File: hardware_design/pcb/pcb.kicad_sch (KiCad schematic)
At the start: 15 parts, among them J1 Eurorack Power, Q1 DMG2305UX, U1 Pico, U2 PCM1808, U5 GY_PCM5102A, U6 APS6404L, U7 LM1117MP-5.0

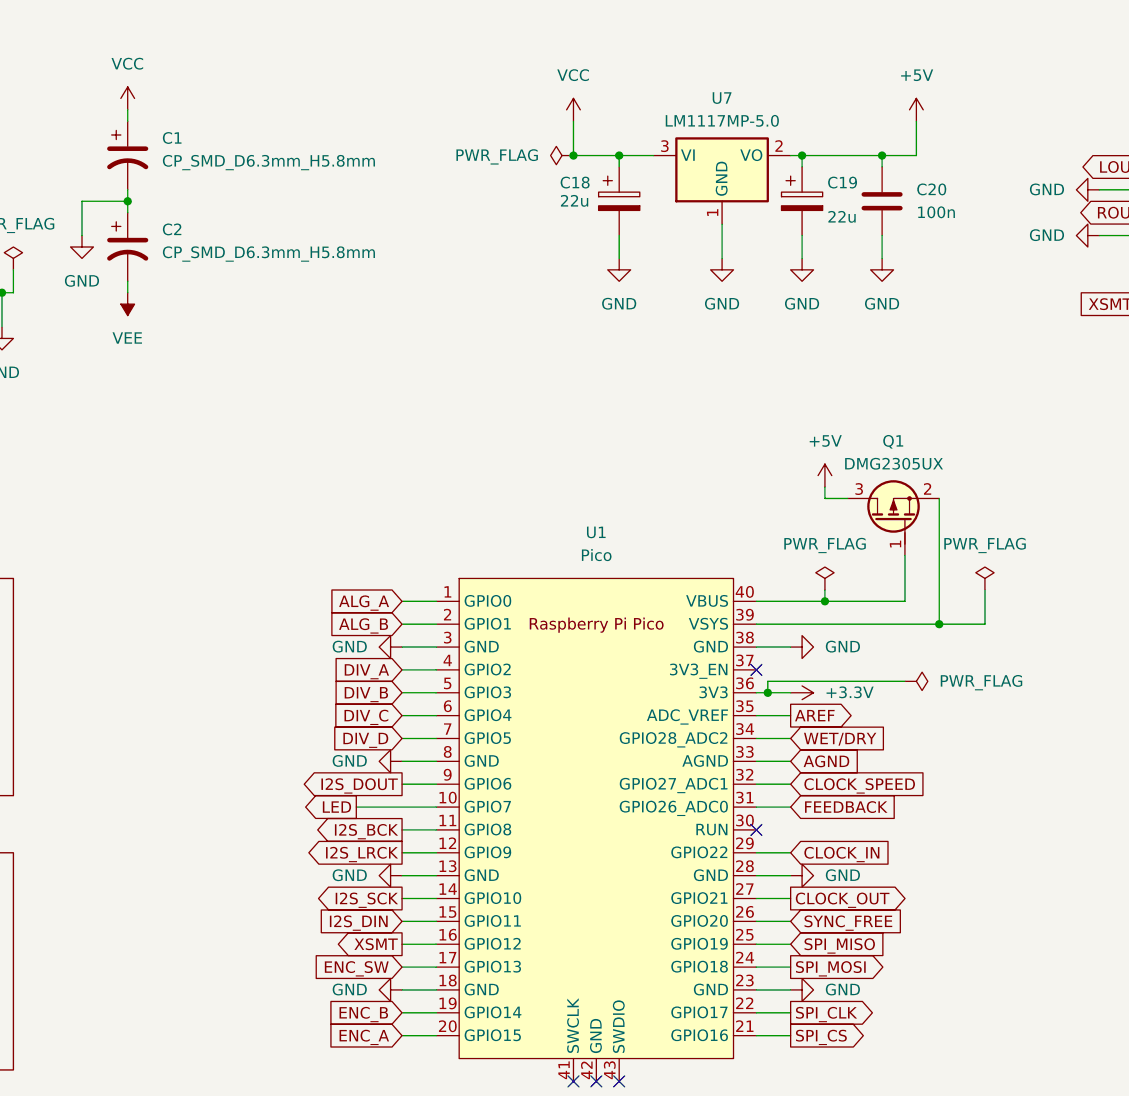
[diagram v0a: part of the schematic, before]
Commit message: Rev 2 schematic & circuit board
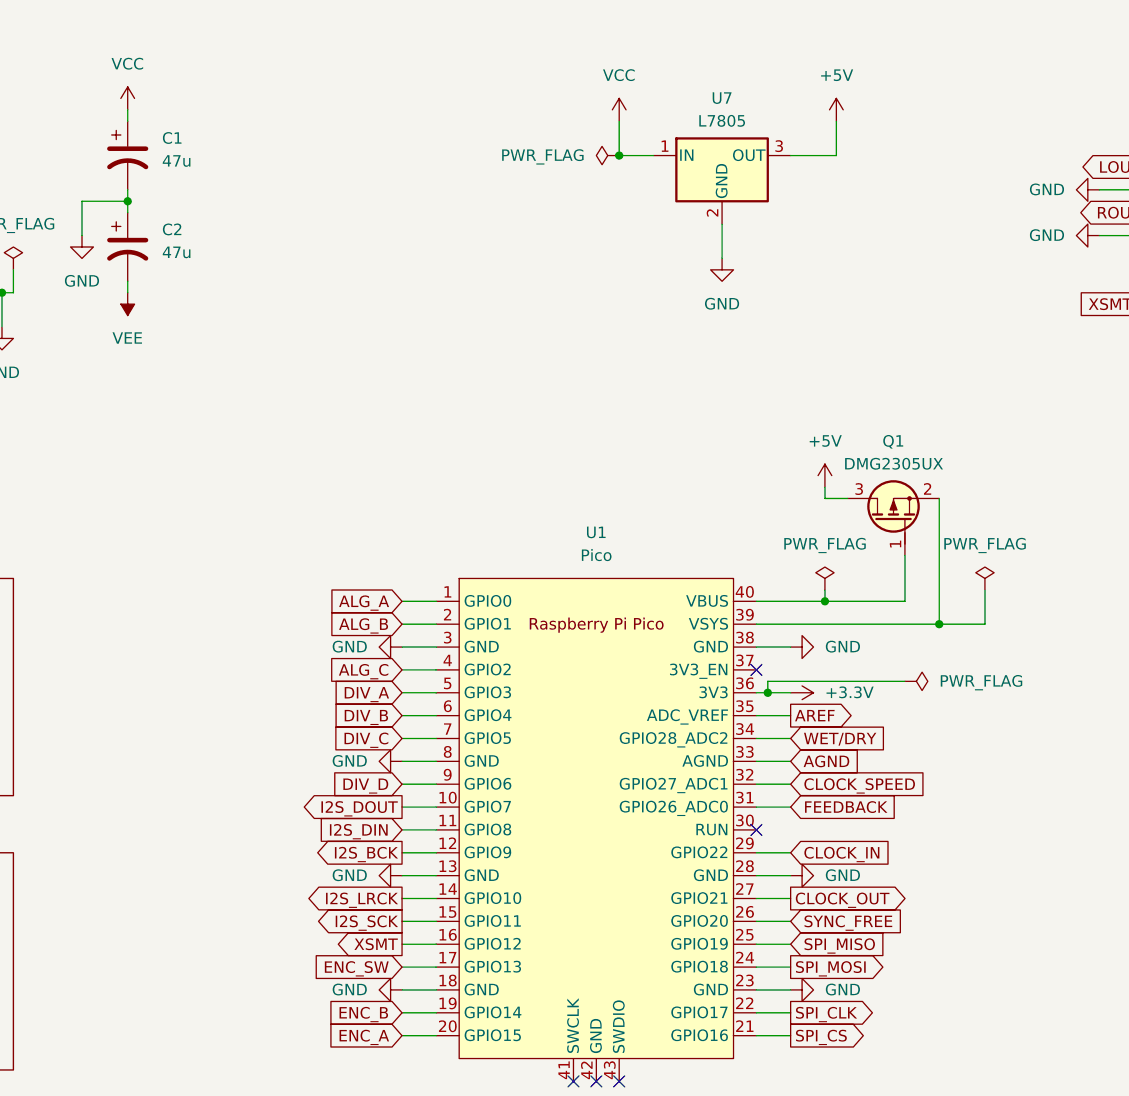
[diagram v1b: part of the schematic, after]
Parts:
- removed C18, C19: 22u, Capacitor_SMD_AKL:CP_Elec_6.3x5.8, symbol Capacitor_AKL:CP_SMD_D6.3mm_H5.8mm
- removed C20: 100n, Capacitor_SMD_AKL:C_0603_1608Metric, symbol Capacitor_AKL:C_0603
- removed U7: LM1117MP-5.0, Package_TO_SOT_SMD:SOT-223-3_TabPin2, symbol Regulator_Linear:LM1117MP-5.0
- added U7: L7805, Package_TO_SOT_SMD:TO-252-2, symbol Regulator_Linear:L7805
- C1, C2: value CP_SMD_D6.3mm_H5.8mm -> 47u
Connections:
- net LED is gone; now on net I2S_DOUT: U1.10 (GPIO7)
- net +5V: now also U7.3 (OUT)
- net DIV_A: now also U1.5 (GPIO3); no longer U1.4 (GPIO2)
- net DIV_B: now also U1.6 (GPIO4); no longer U1.5 (GPIO3)
- net DIV_C: now also U1.7 (GPIO5); no longer U1.6 (GPIO4)
- net DIV_D: now also U1.9 (GPIO6); no longer U1.7 (GPIO5)
- net GND: now also U7.2 (GND)
- net I2S_BCK: now also U1.12 (GPIO9); no longer U1.11 (GPIO8)
- net I2S_DIN: now also U1.11 (GPIO8); no longer U1.15 (GPIO11)
- net I2S_DOUT: no longer U1.9 (GPIO6)
- net I2S_LRCK: now also U1.14 (GPIO10); no longer U1.12 (GPIO9)
- net I2S_SCK: now also U1.15 (GPIO11); no longer U1.14 (GPIO10)
- net VCC: now also U7.1 (IN)
- new net ALG_C: U1.4 (GPIO2)
